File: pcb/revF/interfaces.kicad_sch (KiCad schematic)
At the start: 46 parts, among them CON7 SOUND, CON8 VGA, J5 TAPE IN, J6 TAPE OUT, J7 USB C, U18 ESP-12E, U19 AMS1117-3.3, U20 LM311, U21 TDA1543

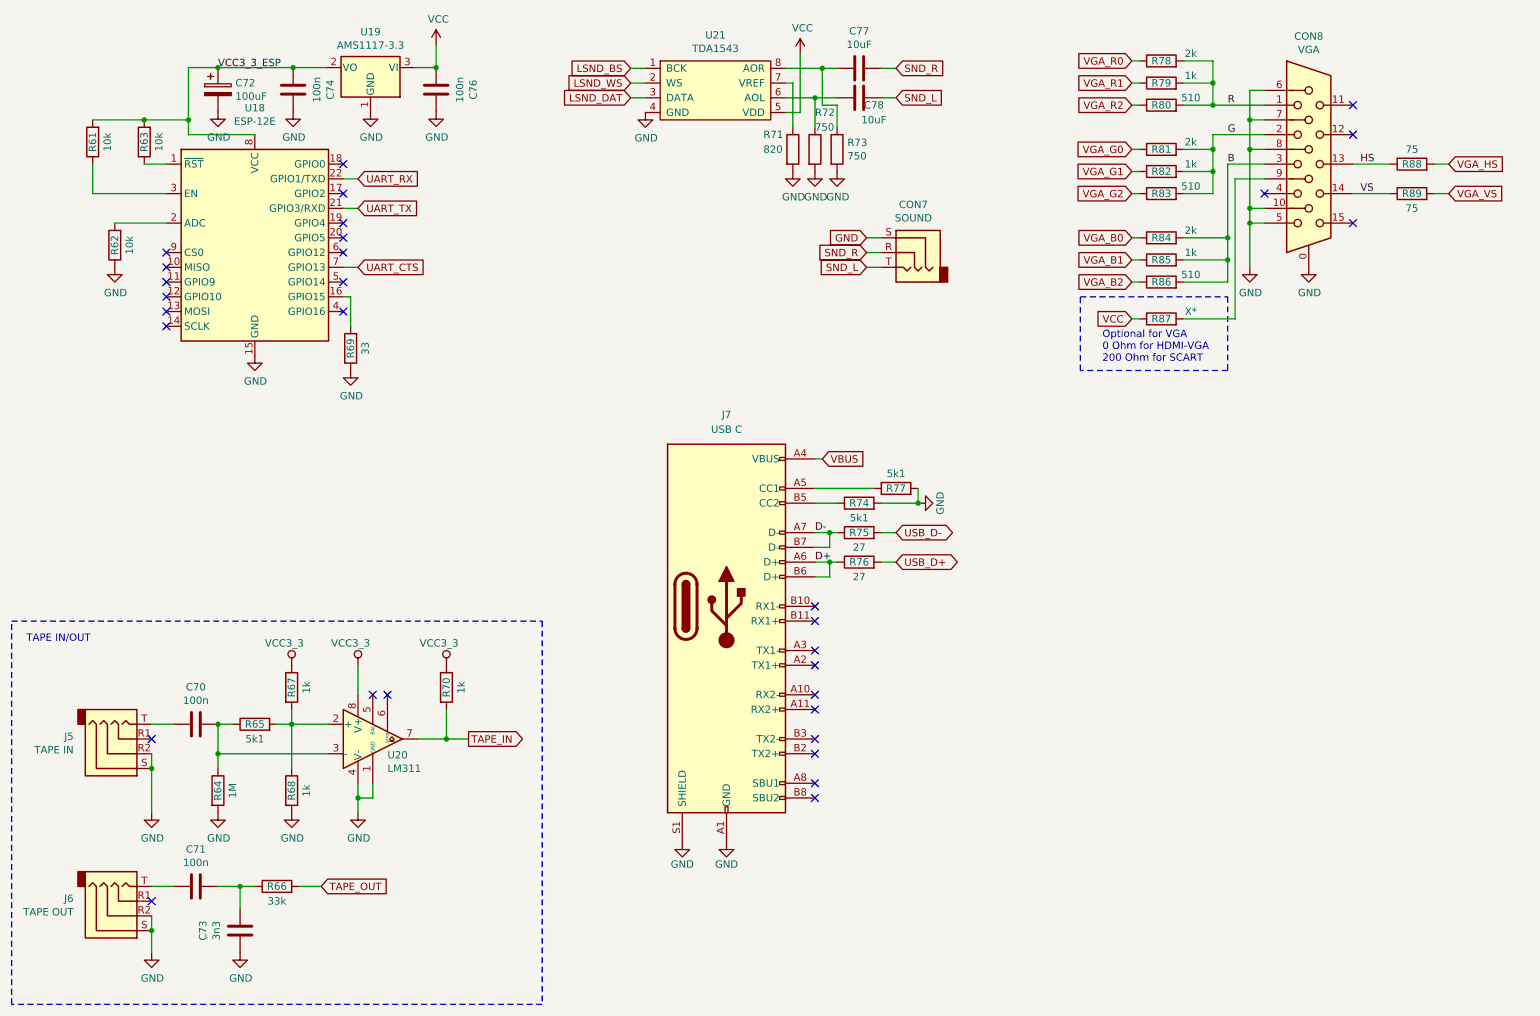
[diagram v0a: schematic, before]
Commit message: revF routed
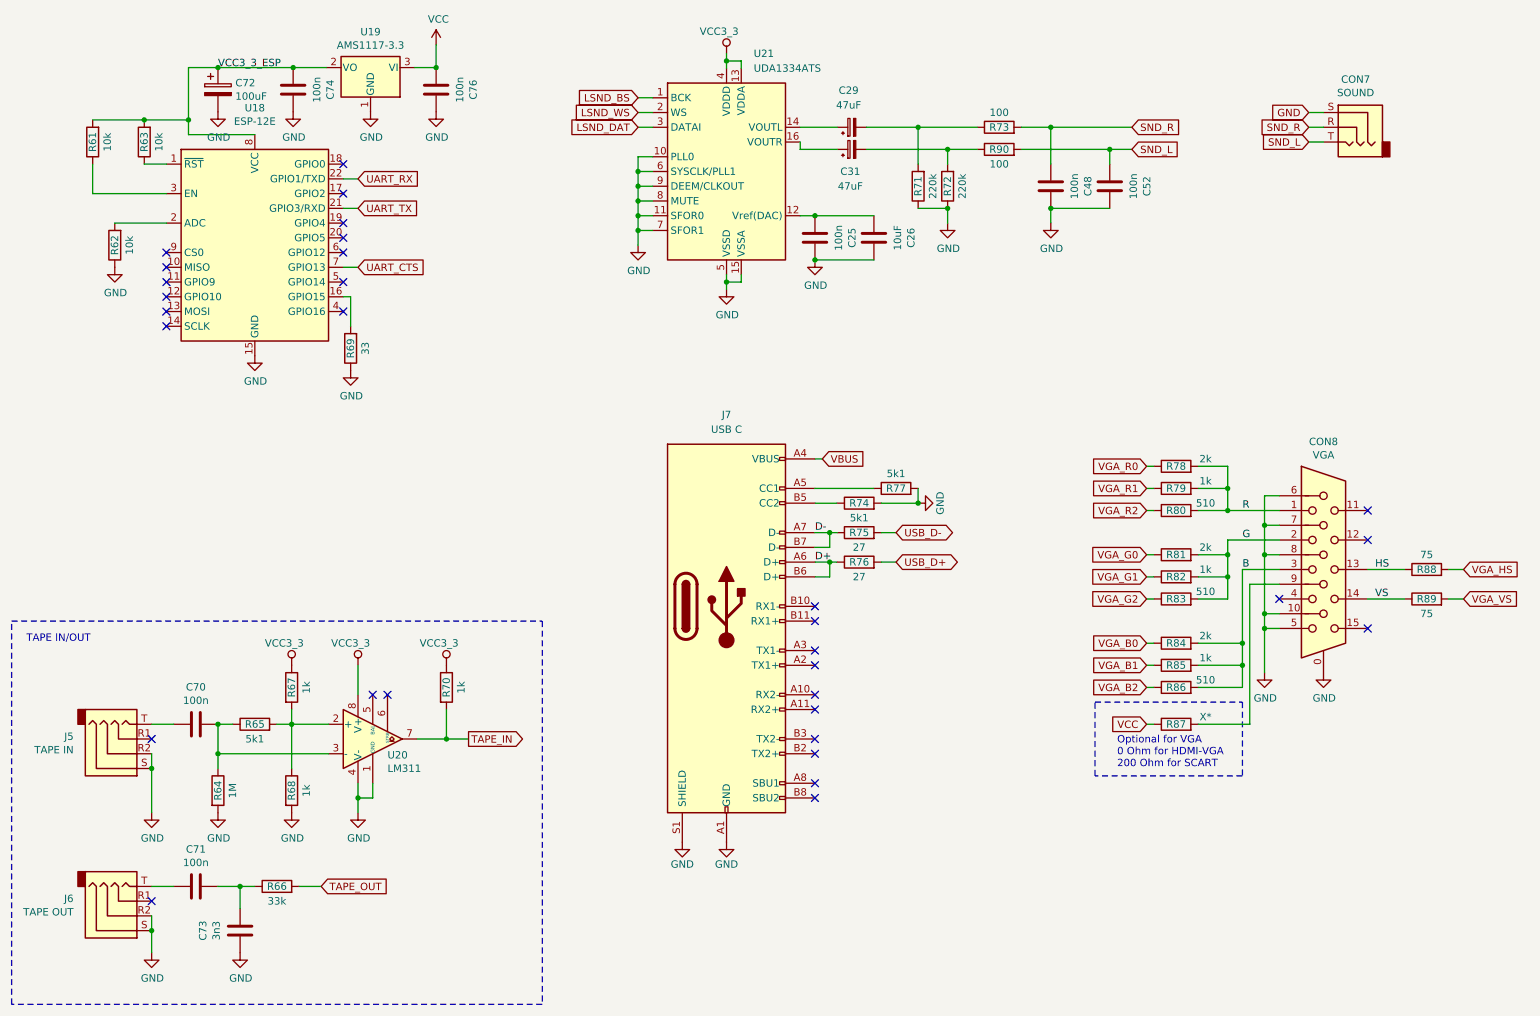
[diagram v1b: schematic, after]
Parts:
- removed C77, C78: 10uF, Capacitor_SMD:C_0805_2012Metric_Pad1.15x1.40mm_HandSolder, symbol Device:C
- removed U21: TDA1543, Package_DIP:DIP-8_W7.62mm, symbol tda1543:TDA1543
- added C25, C48, C52: 100n, Capacitor_SMD:C_0805_2012Metric_Pad1.18x1.45mm_HandSolder, symbol Device:C
- added C26: 10uF, Capacitor_SMD:C_0805_2012Metric_Pad1.18x1.45mm_HandSolder, symbol Device:C
- added C29, C31: 47uF, Capacitor_SMD:CP_Elec_5x5.9, symbol Device:C_Polarized_Small
- added R90: 100, Resistor_SMD:R_0805_2012Metric_Pad1.20x1.40mm_HandSolder, symbol Device:R
- added U21: UDA1334ATS, Package_SO:SSOP-16_4.4x5.2mm_P0.65mm, symbol Audio:UDA1334ATS
- R71: value 820 -> 220k; footprint Resistor_SMD:R_0805_2012Metric_Pad1.15x1.40mm_HandSolder -> Resistor_SMD:R_0805_2012Metric_Pad1.20x1.40mm_HandSolder
- R72: value 750 -> 220k; footprint Resistor_SMD:R_0805_2012Metric_Pad1.15x1.40mm_HandSolder -> Resistor_SMD:R_0805_2012Metric_Pad1.20x1.40mm_HandSolder
- R73: value 750 -> 100; footprint Resistor_SMD:R_0805_2012Metric_Pad1.15x1.40mm_HandSolder -> Resistor_SMD:R_0805_2012Metric_Pad1.20x1.40mm_HandSolder
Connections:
- net GND: now also R71.1, R72.1, C25.2, C26.2, C48.2, C52.2, U21.10 (PLL0), U21.11 (SFOR0), U21.15 (VSSA), U21.5 (VSSD), U21.6 (SYSCLK/PLL1), U21.7 (SFOR1), U21.8 (MUTE), U21.9 (DEEM/CLKOUT); no longer R71.2, R72.2, R73.2
- net LSND_BS: now also U21.1 (BCK)
- net LSND_DAT: now also U21.3 (DATAI)
- net LSND_WS: now also U21.2 (WS)
- net SND_L: now also C52.1, R90.2
- net SND_R: now also R73.2, C48.1
- net VCC3_3: now also U21.13 (VDDA), U21.4 (VDDD)
- net at R73.1: now also R71.2, C29.2
- new net: C25.1, C26.1, U21.12 (Vref(DAC))
- new net: C31.1, U21.16 (VOUTR)
- new net: C31.2, R72.2, R90.1
- new net: C29.1, U21.14 (VOUTL)
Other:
- moved on the sheet: CON7, CON8, R78, R79, R80, R81, R82, R83, R84, R85, R86, R87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
